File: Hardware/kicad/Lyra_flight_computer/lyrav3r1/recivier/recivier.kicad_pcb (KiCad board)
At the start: 4 copper layers, 70 x 80 mm, 87 parts, among them J1 USB_B_Micro, J2 Conn_01x02, J3 Conn_01x02, J4 Screw_Terminal_01x02, J5 Screw_Terminal_01x02, Q1 AO3401A, SW1 K2-1102DP-L3SW-04, SW2 K2-1102DP-L3SW-04, SW3 K2-1102DP-L3SW-04, SW4 K2-1102DP-L3SW-04, SW5 K2-1102DP-L3SW-04, SW6 SW_SPDT, U1 E22-900MM22S, U2 W25Q128JVS, U3 RP2040, U4 TXB0104RGY, U5 PCM5102A, U6 ATGM336H-5N31, U7 LIS3MDLTR, U8 AMS1117-3.3, U9 AMS1117-5.0, X1 SX1M12.000M10F30TNN

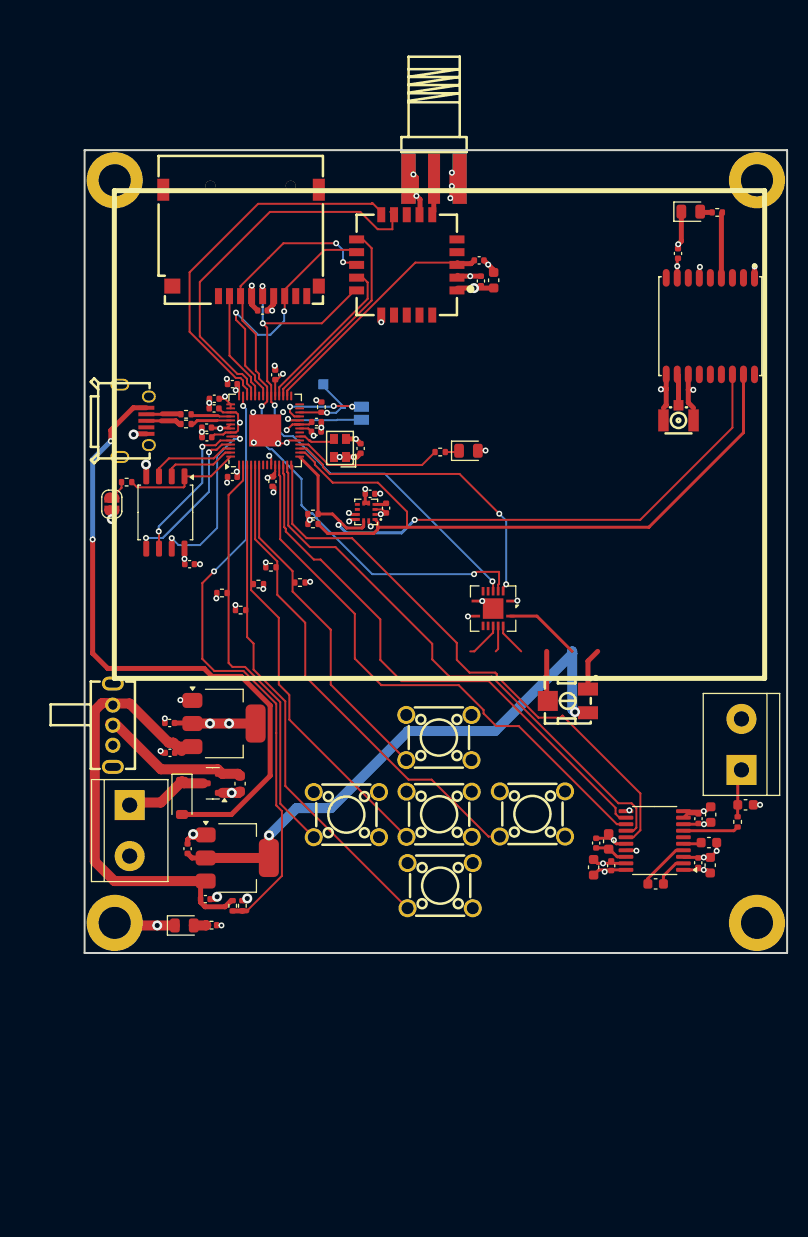
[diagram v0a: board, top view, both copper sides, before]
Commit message: stuffs
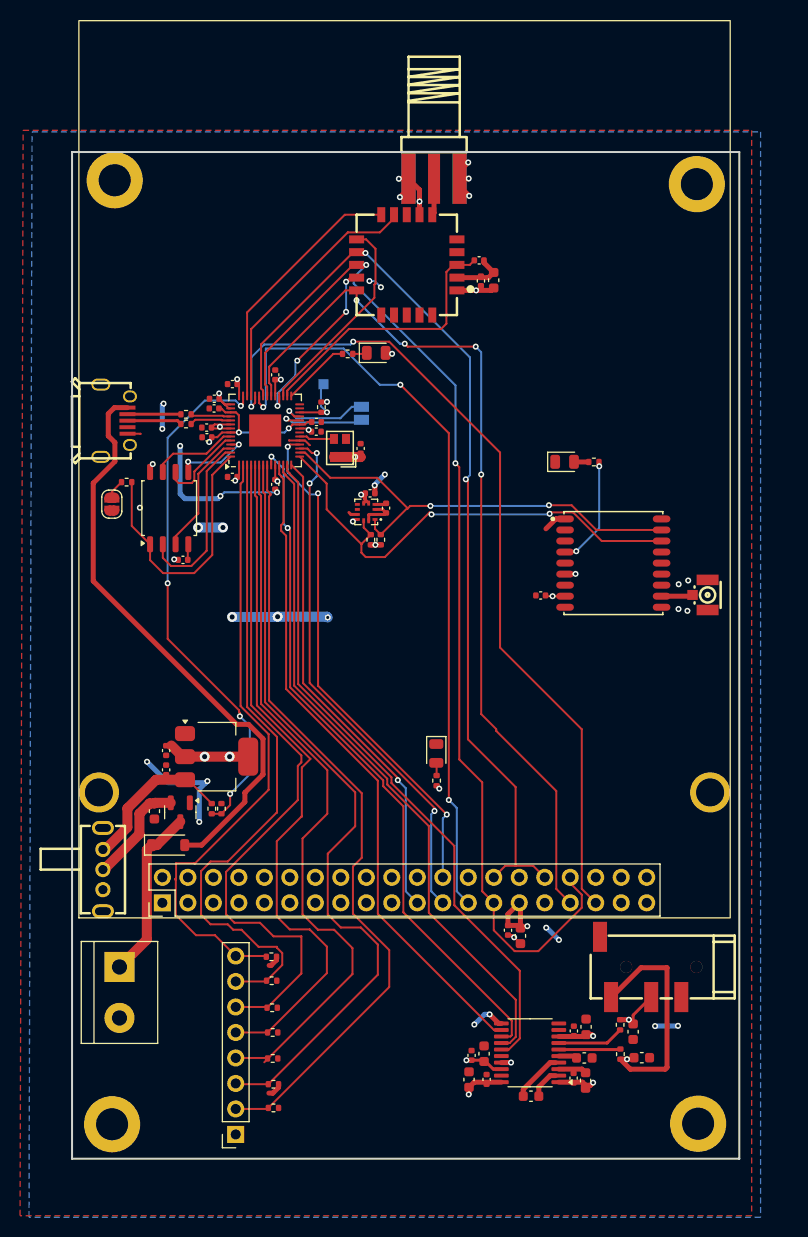
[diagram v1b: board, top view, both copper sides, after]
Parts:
- removed C31, C37, C38: 1u, Capacitor_SMD:C_0402_1005Metric
- removed Card1: TF-115K, .pretty:TF-SMD_TF-115K
- removed J4: Screw_Terminal_01x02, TerminalBlock:TerminalBlock_bornier-2_P5.08mm
- removed RV1: R_Potentiometer, .pretty:RES-ADJ-SMD_3314J
- removed SW1, SW2, SW3, SW4, SW5: K2-1102DP-L3SW-04, .pretty:SW-TH_4P-L6.0-W6.0-P4.50-LS6.5
- removed U4: TXB0104RGY, Package_DFN_QFN:Texas_S-PVQFN-N14
- removed U9: AMS1117-5.0, Package_TO_SOT_SMD:SOT-223-3_TabPin2
- added C16: 100n, Capacitor_SMD:C_0402_1005Metric, F.Cu at (180.9, 124.9)
- added C18: 10u, Capacitor_SMD:C_0603_1608Metric, F.Cu at (182.2, 125.5)
- added C19: 2u2, Capacitor_SMD:C_0603_1608Metric, F.Cu at (194.3, 137.6)
- added D5: ER-TFT032A3-3, .pretty:R-TFT032IPS-3.2, F.Cu at (146.5, 122.2)
- added J6: Conn_01x08, Connector_PinSocket_2.54mm:PinSocket_1x08_P2.54mm_Vertical, F.Cu at (153.8, 145.3)
- added J8: AudioJack4, .pretty:AUDIO-SMD_PJ-320D, F.Cu at (194.1, 128.6)
- added R18: 5.1k, Resistor_SMD:R_0402_1005Metric, F.Cu at (157.4, 129.9)
- added R19: 5.1k, Resistor_SMD:R_0402_1005Metric, F.Cu at (157.4, 127.6)
- added R20: 470, Resistor_SMD:R_0402_1005Metric, F.Cu at (192.1, 137.3)
- moved R13 52.4 mm to (157.6, 142.6)
- moved R11 49.2 mm to (157.6, 140.3), turned to 0 degrees
- moved R12 47.3 mm to (157.5, 137.7)
- moved R8 46.4 mm to (157.5, 135.1), turned to 0 degrees
- moved R10 39.7 mm to (157.4, 132.6), turned to 0 degrees
- moved C17 36.7 mm to (184.2, 91.6), turned to 180 degrees
- moved D2 30.4 mm to (173.8, 107.3), turned to -90 degrees
- moved D1 27.9 mm to (186.6, 78.2)
- moved R7 27.7 mm to (189.5, 78.3)
- moved R14 26.7 mm to (173.8, 110.0), turned to -90 degrees
- moved U6 25.5 mm to (191.4, 88.3), turned to 90 degrees
- moved C30 25.2 mm to (193.4, 135.0), turned to -90 degrees
- moved C27 24.8 mm to (188.7, 139.9)
- moved C26 24.8 mm to (187.5, 139.6)
- moved C21 24.8 mm to (188.5, 137.6)
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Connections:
- net /AUDIOOUT renamed /AUDIOOUT R
- U3 pad 11: /BCK -> /SCK
- U3 pad 12: /SCK -> /DIN
- U3 pad 13: /DIN -> /LRCK
- U3 pad 14: /LRCK -> /LCD RST
- U3 pad 18: /LEDINDICATION -> /LCD D/C
- U3 pad 2: /BUTTON2 -> /BUTTON7
- U3 pad 29: unconnected-(U3-GPIO18-Pad29) -> /LEDINDICATION
- U3 pad 3: /BUTTON5 -> /BUTTON6
- U3 pad 37: unconnected-(U3-GPIO25-Pad37) -> /LCD /WR
- U3 pad 4: /BUTTON3 -> /BUTTON5
- U3 pad 6: /BUTTON1 -> /BUTTON3
- U3 pad 7: unconnected-(U3-GPIO5-Pad7) -> /BUTTON2
- U3 pad 8: unconnected-(U3-GPIO6-Pad8) -> /BUTTON1
- U3 pad 9: unconnected-(U3-GPIO7-Pad9) -> /BCK
- U5 pad 6: unconnected-(U5-OUTL-Pad6) -> Net-(U5-OUTL)
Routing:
- net /LCD /WR: track 0.00 -> 76.4 mm, vias 0 -> 3
- net /SD_CS: track 11.0 -> 85.0 mm, vias 0 -> 2
- net /BUTTON6: track 0.00 -> 66.4 mm
- net /MISO: track 27.7 -> 92.2 mm
- net +5V: track 62.3 -> 0.00 mm, vias 2 -> 0
- net /BUTTON7: track 0.00 -> 61.9 mm
- net /LCD D/C: track 0.00 -> 51.6 mm, vias 0 -> 3
- net /LCD RST: track 0.00 -> 48.8 mm, vias 0 -> 1
- net /BUTTON1: track 35.6 -> 78.2 mm
- net /MOSI: track 64.9 -> 104.6 mm, vias 4 -> 2
- net /BUTTON2: track 41.9 -> 77.7 mm
- net /SCLK: track 55.5 -> 89.0 mm
- net +BATT: track 46.1 -> 15.8 mm
- net /BUTTON3: track 43.5 -> 73.2 mm
- net /SCL: track 68.6 -> 45.0 mm, vias 0 -> 2
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- added copper zone on B.Cu, net +3.3VA
- added copper zone on F.Cu, net GND
- removed copper zone on In2.Cu, net +3.3VA
- removed copper zone on In1.Cu, net GND
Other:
- board size 70 x 80 mm -> 66.5 x 100.3 mm
- copper layers 4 -> 2

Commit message: post order omcmit
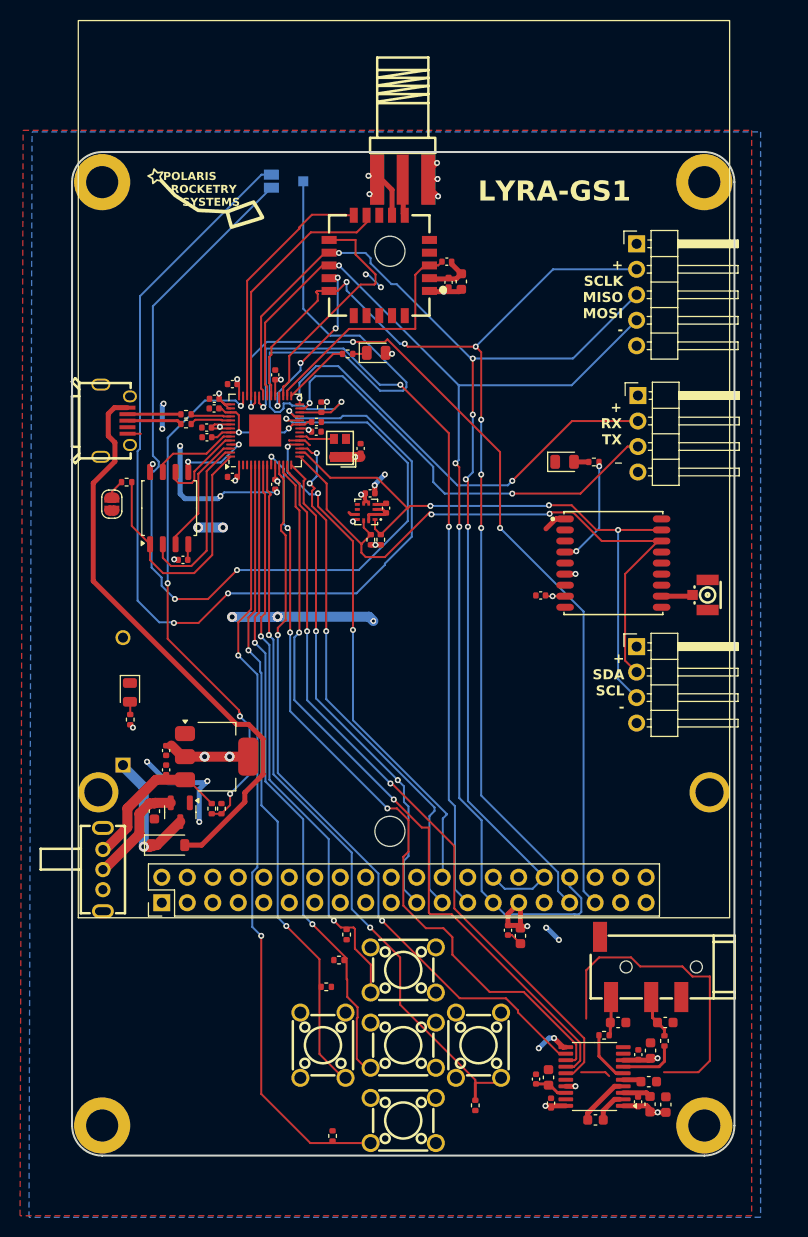
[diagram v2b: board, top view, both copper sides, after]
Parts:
- removed J5: Screw_Terminal_01x02, TerminalBlock:TerminalBlock_bornier-2_P5.08mm
- removed J6: Conn_01x08, Connector_PinSocket_2.54mm:PinSocket_1x08_P2.54mm_Vertical
- removed R18, R19: 5.1k, Resistor_SMD:R_0402_1005Metric
- added BT1: Battery, SamacSys_Parts:12BH349GR, B.Cu at (142.6, 108.5)
- added G***: LOGO, LOGO, F.Cu at (150.7, 54.6)
- added J10: Conn_01x05, Connector_PinHeader_2.54mm:PinHeader_1x05_P2.54mm_Horizontal, F.Cu at (193.7, 56.5)
- added J4: Conn_01x04, Connector_PinHeader_2.54mm:PinHeader_1x04_P2.54mm_Horizontal, F.Cu at (193.7, 96.7)
- added J7: Conn_01x04, Connector_PinHeader_2.54mm:PinHeader_1x04_P2.54mm_Horizontal, F.Cu at (193.9, 71.6)
- added SW1: K2-1102DP-L3SW-04, .pretty:SW-TH_4P-L6.0-W6.0-P4.50-LS6.5, F.Cu at (170.5, 128.9)
- added SW2: K2-1102DP-L3SW-04, .pretty:SW-TH_4P-L6.0-W6.0-P4.50-LS6.5, F.Cu at (162.5, 136.4)
- added SW3: K2-1102DP-L3SW-04, .pretty:SW-TH_4P-L6.0-W6.0-P4.50-LS6.5, F.Cu at (170.5, 136.4)
- added SW4: K2-1102DP-L3SW-04, .pretty:SW-TH_4P-L6.0-W6.0-P4.50-LS6.5, F.Cu at (178.0, 136.4)
- added SW5: K2-1102DP-L3SW-04, .pretty:SW-TH_4P-L6.0-W6.0-P4.50-LS6.5, F.Cu at (170.5, 143.9)
- R16: value 1k -> 15k
- moved D2 31.1 mm to (143.3, 101.2)
- moved R14 31.1 mm to (143.3, 103.9)
- moved J2 24.8 mm to (157.4, 50.3)
- moved R8 21.5 mm to (177.7, 142.4), turned to -90 degrees
- moved TP1 20.3 mm to (160.5, 50.3)
- moved C29 19.8 mm to (196.7, 142.3)
- moved R13 18.7 mm to (164.8, 125.3), turned to -90 degrees
- moved R10 14.1 mm to (163.4, 145.4), turned to 90 degrees
- moved R12 11.8 mm to (164.1, 127.9), turned to 180 degrees
- moved R11 11.0 mm to (162.8, 130.6)
- moved C28 6.84 mm to (185.2, 142.1)
- moved C27 6.84 mm to (195.1, 142.3)
- moved C20 6.84 mm to (189.6, 143.8)
- moved C21 6.84 mm to (195.0, 140.0)
- moved C22 6.84 mm to (185.0, 139.6)
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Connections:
- U3 pad 2: /BUTTON7 -> unconnected-(U3-GPIO0-Pad2)
- U3 pad 27: unconnected-(U3-GPIO16-Pad27) -> /UART0 TX
- U3 pad 28: unconnected-(U3-GPIO17-Pad28) -> /UART0 RX
- U3 pad 3: /BUTTON6 -> unconnected-(U3-GPIO1-Pad3)
- U3 pad 5: /BUTTON4 -> /BUTTON2
- U3 pad 7: /BUTTON2 -> /BUTTON1
- U3 pad 8: /BUTTON1 -> /BUTTON4
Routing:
- net /SWD: track 9.25 -> 103.7 mm, vias 1 -> 3
- net /SWCLK: track 9.17 -> 95.1 mm, vias 1 -> 3
- net /BUTTON6: track 66.4 -> 0.00 mm
- net /BUTTON7: track 61.9 -> 0.00 mm
- net /RUN: track 5.87 -> 60.4 mm
- net /UART0 RX: track 0.00 -> 44.2 mm, vias 0 -> 2
- net /UART0 TX: track 0.00 -> 44.0 mm, vias 0 -> 2
- net (no net): track 0.00 -> 34.9 mm
- net /MISO: track 92.2 -> 115.6 mm, vias 2 -> 5
- net /SCLK: track 89.0 -> 110.5 mm, vias 4 -> 6
- net /BUTTON1: track 78.2 -> 58.2 mm, vias 0 -> 2
- net /AUDIOOUT L: track 23.3 -> 3.59 mm, vias 1 -> 0
- net /SCL: track 45.0 -> 62.5 mm, vias 2 -> 3
- net /SDA: track 48.6 -> 63.7 mm
- net /MOSI: track 104.6 -> 119.4 mm, vias 2 -> 3
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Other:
- board size 66.5 x 100.3 mm -> 66 x 100 mm
- board text added: "+ RX TX _"
- board text added: "+ SCLK MISO MOSI -"
- board text added: "+ SDA SCL -"
- board text added: "LYRA-GS1"
- board text added: "POLARIS ROCKETRY SYSTEMS"
